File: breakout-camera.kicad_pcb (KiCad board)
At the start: 2 copper layers, 36.1 x 28.4 mm, 88 parts, among them P1 CONN_01X02, P10 CONN_01X14, P11 CONN_01X12, P2 CONN_01X18, P3 CONN_01X18, P8 CONN_01X06, P9 CONN_01X02, Q1 2SC5095, Q2 MT3S20TU, Q3 2SC5095, Q4 MT3S20TU, U1 TPS2420, U10 ICX825AQA, U11 ADDI7013, U2 LT3487, U3 TPS63002, U7 TPS56x200, U8 LMZ10500, U9 CXD3400N

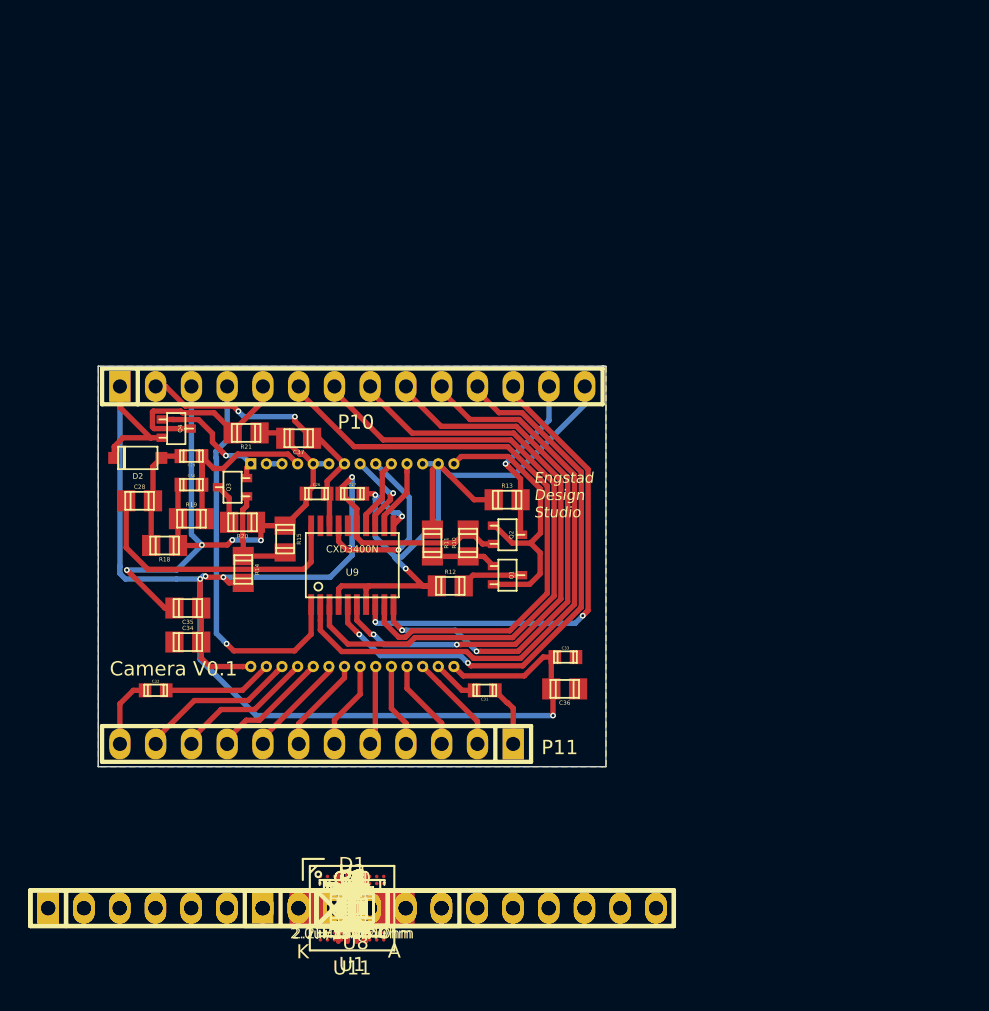
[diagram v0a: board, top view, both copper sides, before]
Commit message: lots of work
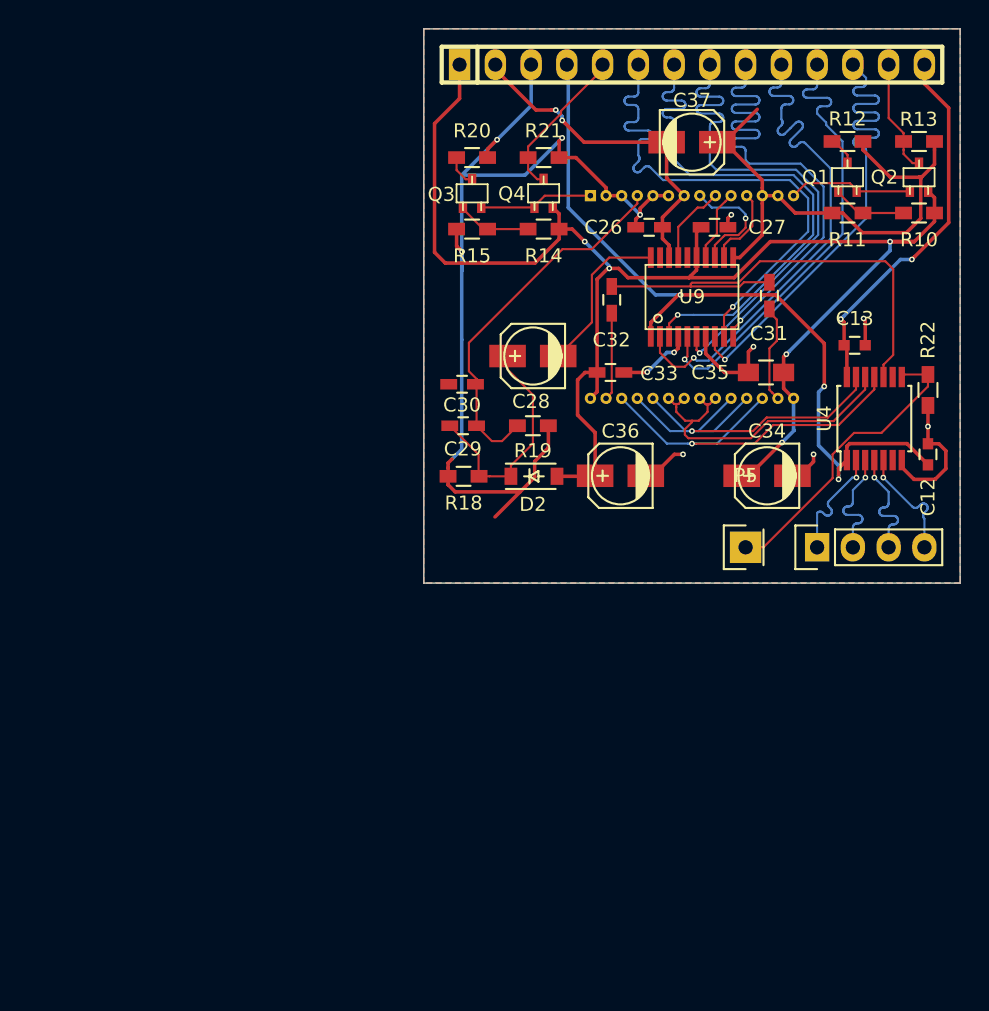
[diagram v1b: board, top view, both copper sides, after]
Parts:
- removed C1, C2, C6: 1.0uF, Capacitors_SMD:C_0805_HandSoldering
- removed C10: 0.1uF, Capacitors_SMD:C_0805_HandSoldering
- removed C11: 10uF, Capacitors_SMD:C_0805_HandSoldering
- removed C14: 10.0F/3.0mOhm, w_smd_cap:c_0603
- removed C15: 10.0F/9Mohm, w_smd_cap:c_0603
- removed C16: 470pF, w_smd_cap:c_0603
- removed C20: 100nF, w_smd_cap:c_0603
- removed C21: 10.0uF/9.0Mohm, w_smd_cap:c_0603
- removed C25: 47F/3Mohm, w_smd_cap:c_0603
- removed C3, C5: 47pF, Capacitors_SMD:C_0805_HandSoldering
- removed C38, C39, C40, C41, C42, C43, C44, C45, C46: 0.1uF, w_smd_cap:c_0603
- removed C4: 2.20uF/2.80Mohm, w_smd_cap:c_0603
- removed C47: 4.7uF, w_smd_cap:c_0603
- removed C48, C49: 0.1u, w_smd_cap:c_0603
- removed C7: 100nF, Capacitors_SMD:C_0805_HandSoldering
- removed C8: 1.0F/11mOhm, Capacitors_SMD:C_0805_HandSoldering
- removed C9: 4.7uF, Capacitors_SMD:C_0805_HandSoldering
- removed D1: 9V/5W, Diodes_SMD:Diode-SMB_Handsoldering
- removed L1, L2: 15uH, w_smd_inductors:inductor_smd_0805
- removed L3: 2.0uH/0.024Ohm, w_smd_inductors:inductor_smd_0805
- removed L4: 10uH, w_smd_inductors:inductor_smd_0805
- removed L8: 2.2H/13.0mOhm, w_smd_inductors:inductor_smd_0805
- removed P1: CONN_01X02, w_pin_strip:pin_strip_2
- removed P11: CONN_01X12, w_pin_strip:pin_strip_12
- removed P2, P3: CONN_01X18, w_pin_strip:pin_strip_18
- removed P8: CONN_01X06, w_pin_strip:pin_socket_6
- removed P9: CONN_01X02, w_pin_strip:pin_socket_2
- removed R1, R3: 10.0kE, Resistors_SMD:R_0805_HandSoldering
- removed R16: 13.7kE, w_smd_resistors:r_0805
- removed R17: 10.0kE, w_smd_resistors:r_0805
- removed R2, R7: 324kE, w_smd_resistors:r_0603
- removed R4: 51.1kE, Resistors_SMD:R_0805_HandSoldering
- removed R5: 68.1kE, Resistors_SMD:R_0805_HandSoldering
- removed R6: 53.6kE, Resistors_SMD:R_0805_HandSoldering
- removed R8: 80.6kE, w_smd_resistors:r_0805
- removed R9: 105kE, w_smd_resistors:r_0805
- removed U1: TPS2420, camera:S-PVQFN-N16
- removed U11: ADDI7013, camera:csp-bga-bc-76-3
- removed U2: LT3487, w_smd_qfn:dfn10-3x3
- removed U3: TPS63002, Housings_DFN_QFN:DFN-10-1EP_3x3mm_Pitch0.5mm
- removed U7: TPS56x200, w_smd_trans:sot23-6
- removed U8: LMZ10500, camera:llp-8
- added C12: 0.1u, Capacitors_SMD:C_0603, F.Cu at (93.0, 74.7)
- added C13: 0.1u, Capacitors_SMD:C_0603, F.Cu at (87.8, 66.9)
- added P4: CONN_01X04, Socket_Strips:Socket_Strip_Straight_1x04, F.Cu at (85.1, 81.3)
- added P5: CONN_01X01, Socket_Strips:Socket_Strip_Straight_1x01, F.Cu at (80.0, 81.3)
- added R22: 10.0k, Resistors_SMD:R_0603_HandSoldering, F.Cu at (93.0, 70.1)
- added U4: TXB0104, Housings_SSOP:TSSOP-14_4.4x5mm_Pitch0.65mm, F.Cu at (89.2, 72.1)
- C26, C27, C29, C30, C31, C32, C33: footprint w_smd_cap:c_0603 -> Capacitors_SMD:C_0603_HandSoldering
- C28, C34, C36, C37: footprint w_smd_cap:c_0805 -> Capacitors_SMD:c_elec_4x5.3
- C35: footprint w_smd_cap:c_0805 -> Capacitors_SMD:C_0805_HandSoldering
- D2: footprint w_smd_diode:sod123 -> Diodes_SMD:SOD-123
- R10, R11, R12, R13, R14, R15, R18, R19, R20, R21: footprint w_smd_resistors:r_0805 -> Resistors_SMD:R_0603_HandSoldering
- moved C35 44.4 mm to (81.5, 68.9), turned to 0 degrees
- moved C34 42.8 mm to (81.5, 76.2), turned to 180 degrees
- moved C32 42.7 mm to (70.5, 63.7), turned to 90 degrees
- moved R12 42.3 mm to (87.2, 52.5)
- moved R10 39.7 mm to (92.3, 57.5), turned to 180 degrees
- moved R13 38.8 mm to (92.3, 52.5)
- moved Q2 38.7 mm to (92.3, 55.0), turned to 0 degrees
- moved R11 37.7 mm to (87.2, 57.5), turned to 180 degrees
- moved Q1 37.2 mm to (87.2, 55.0), turned to 0 degrees
- moved C37 35.0 mm to (76.2, 52.5), turned to 0 degrees
- moved C31 34.6 mm to (81.7, 63.4), turned to 90 degrees
- moved P10 33.2 mm to (76.2, 47.0)
- moved R14 32.2 mm to (65.7, 58.7), turned to 180 degrees
- moved C27 31.9 mm to (77.8, 58.5)
- moved Q4 31.0 mm to (65.7, 56.1), turned to 0 degrees
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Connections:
- C26 pad 2: /camera/GND -> GND
- C27 pad 1: /camera/GND -> /camera/12V
- C27 pad 2: /camera/12V -> GND
- C30 pad 2: /camera/GND -> GND
- C31 pad 1: Net-(C31-Pad1) -> /camera/RG_1
- C31 pad 2: /camera/RG_1 -> /camera/ORG
- C32 pad 1: Net-(C32-Pad1) -> /camera/RG_2
- C32 pad 2: /camera/RG_2 -> /camera/ORG
- C33 pad 1: /camera/GND -> GND
- C34 pad 2: /camera/GND -> GND
- C35 pad 1: /camera/GND -> GND
- C36 pad 2: /camera/GND -> GND
- C37 pad 1: /camera/GND -> GND
- P10 pad 14: /camera/GND -> /camera/5V0
- P10 pad 3: /camera/GND -> GND
- R11 pad 2: /camera/GND -> GND
- R12 pad 2: /camera/GND -> GND
- R13 pad 2: /camera/GND -> GND
- R15 pad 2: /camera/GND -> GND
- R18 pad 2: /camera/GND -> GND
- R19 pad 2: /camera/GND -> GND
- R20 pad 2: /camera/GND -> GND
- R21 pad 2: /camera/GND -> GND
- U10 pad 12: /camera/GND -> GND
- U10 pad 13: /camera/GND -> GND
- U10 pad 16: Net-(C31-Pad1) -> /camera/RG_1
- U10 pad 19: /camera/H1T_1 -> /camera/H1S_1
- U10 pad 2: /camera/GND -> GND
- U10 pad 21: /camera/H2T_1 -> /camera/H2S_1
- U10 pad 22: /camera/H2T_2 -> /camera/H2S_1
- U10 pad 23: /camera/H2S_2 -> /camera/H2S_1
- U10 pad 24: /camera/H1T_2 -> /camera/H1S_1
- U10 pad 25: /camera/H1S_2 -> /camera/H1S_1
- U10 pad 26: /camera/LH1_2 -> /camera/LH1_1
- U10 pad 27: Net-(C32-Pad1) -> /camera/RG_2
- U10 pad 3: /camera/GND -> GND
- U10 pad 5: /camera/GND -> GND
- U10 pad 6: /camera/GND -> GND
- U9 pad 11: /camera/GND -> GND
- U9 pad 4: /camera/GND -> GND
- U9 pad 7: /camera/GND -> GND
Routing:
- net GND: track 0.00 -> 140.8 mm, vias 0 -> 12
- net /camera/GND: track 104.5 -> 0.00 mm, vias 7 -> 0
- net /camera/ORG: track 0.00 -> 34.7 mm
- net /camera/3V3: track 27.7 -> 55.8 mm, vias 1 -> 3
- net /camera/5V0: track 0.00 -> 26.7 mm, vias 0 -> 2
- net /camera/H1S_1: track 6.52 -> 30.0 mm, vias 0 -> 1
- net /camera/ENH: track 0.00 -> 21.5 mm
- net /camera/LH1_1: track 7.11 -> 28.3 mm, vias 0 -> 1
- net /camera/H2S_1: track 5.66 -> 23.2 mm
- net /camera/SUB: track 14.5 -> 26.6 mm
- net /camera/VOUT1: track 20.7 -> 8.93 mm
- net /camera/LH1_2: track 11.5 -> 0.00 mm
- net /camera/H1S_2: track 10.0 -> 0.00 mm
- net Net-(C28-Pad1): track 7.96 -> 16.8 mm
- net /camera/H1T_2: track 8.59 -> 0.00 mm
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- added copper zone on B.Cu, net GND
- added copper zone on F.Cu, net GND
- removed copper zone on B.Cu, net /camera/GND
- removed copper zone on F.Cu, net /camera/GND
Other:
- board size 36.1 x 28.4 mm -> 38.1 x 39.4 mm
- net class Power added: clearance 0.1016, trace_width 0.254, via_dia 0.4064, via_drill 0.2032
- board text removed: "Camera V0.1"
- board text removed: "Engstad Design Studio"
